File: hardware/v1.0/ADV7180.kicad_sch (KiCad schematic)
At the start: 48 parts, among them J5 Conn_01x03, J6 Conn_01x03, J7 Conn_01x04, J8 Conn_01x34, U13 TLV75718PDRV, U2 CH32V003JxMx, U4 ADV7180BCP32Z-RL, U5 TLV62585, Y1 28.63636MHz

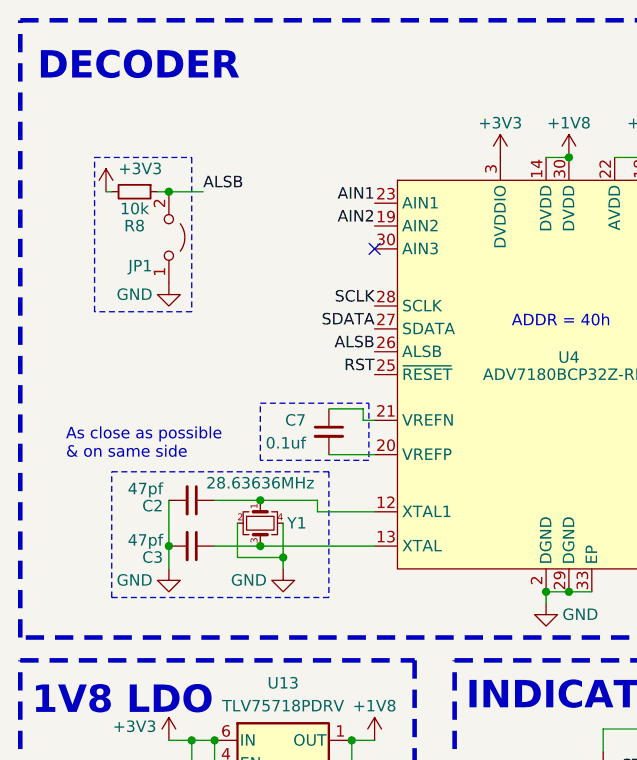
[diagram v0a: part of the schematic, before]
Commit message: changes
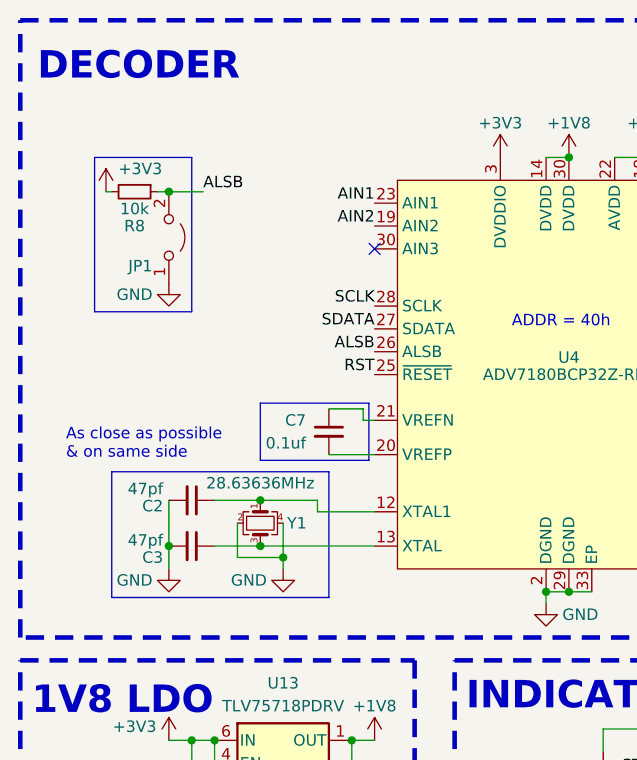
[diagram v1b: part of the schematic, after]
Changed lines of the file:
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@@
 		(stroke
 			(width 0)
-			(type dash)
+			(type solid)
 		)
 		(fill
@@
 		(stroke
 			(width 0)
-			(type dash)
+			(type solid)
 		)
 		(fill
@@
 		(stroke
 			(width 0)
-			(type dash)
+			(type solid)
 		)
 		(fill
